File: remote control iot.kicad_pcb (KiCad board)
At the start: 2 copper layers, 97 x 122.5 mm, 13 parts, among them K1 Fujitsu_FTR-LYAA005x, Q1 BC547, SW2 SW_Push, U1 Olimex_MOD-WIFI-ESP8266-DEV, U2 AMS1117-3.3

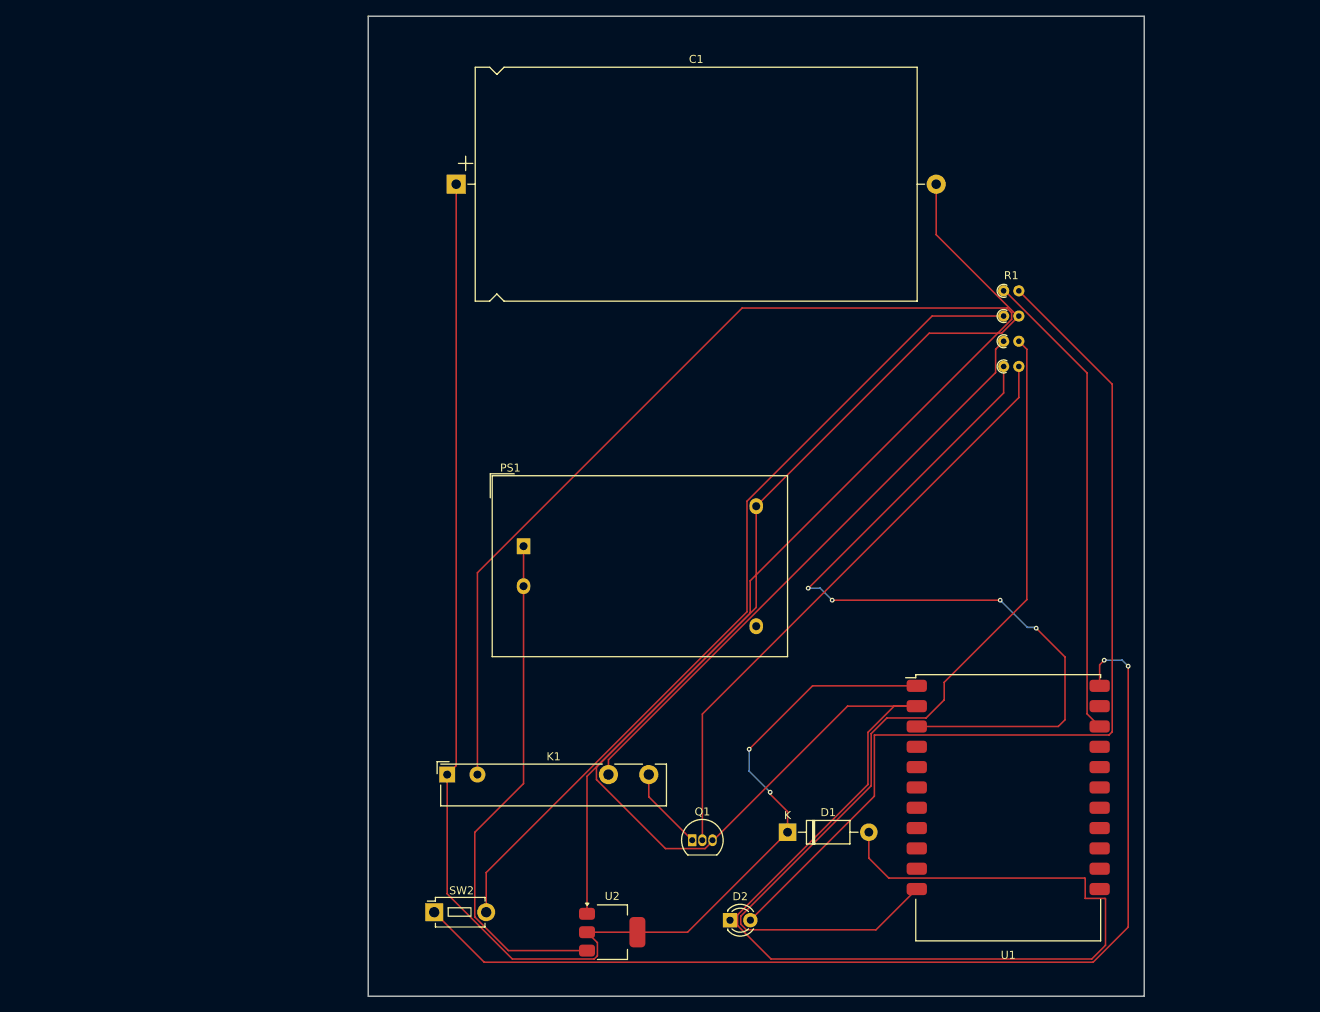
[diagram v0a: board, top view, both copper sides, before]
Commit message: Add files via upload
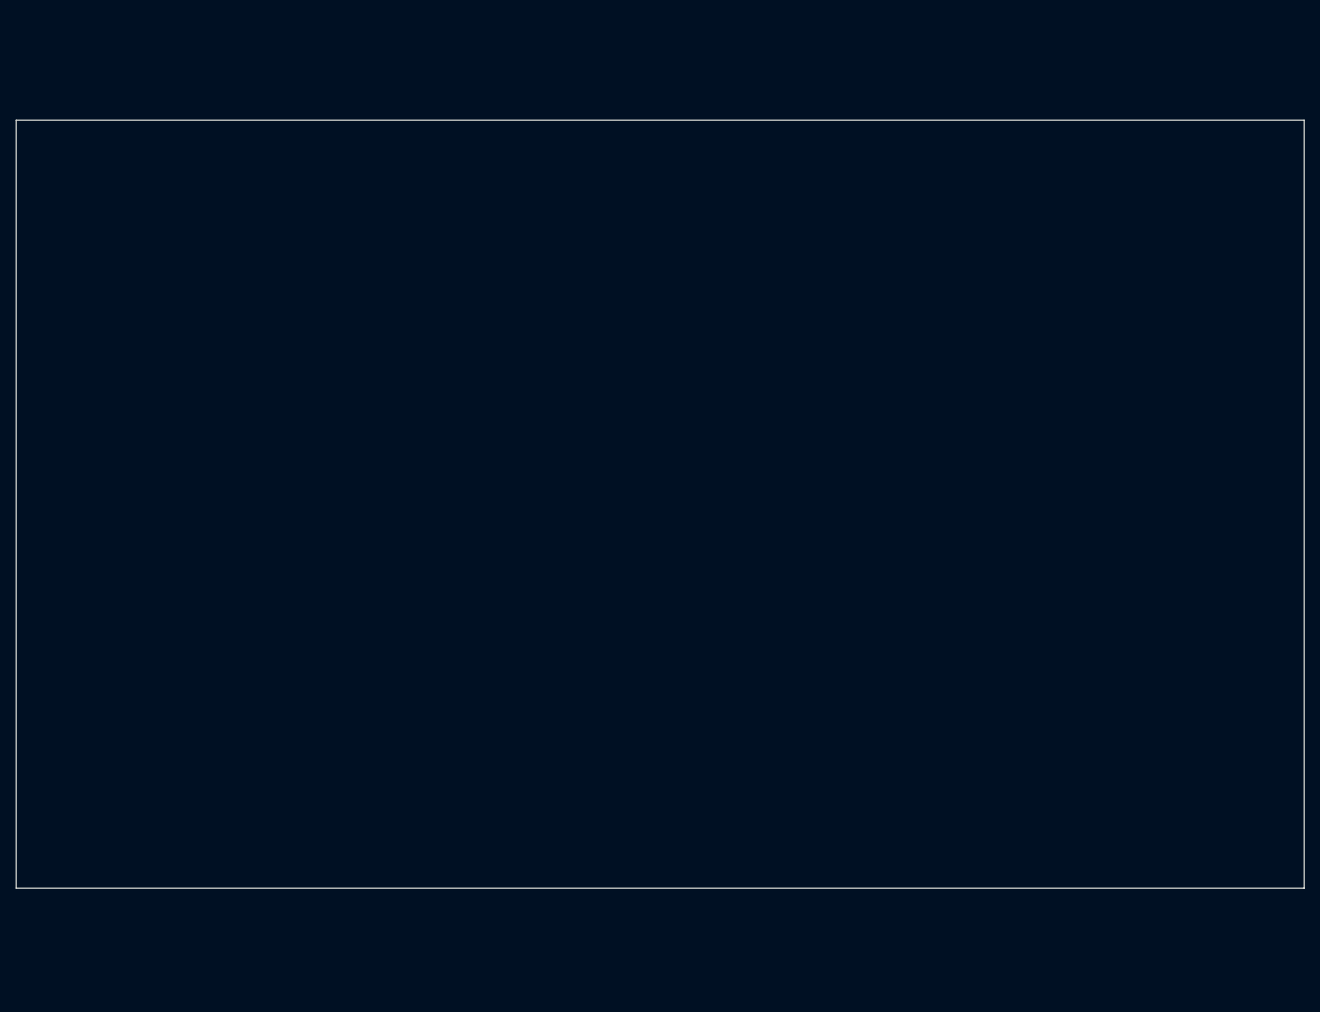
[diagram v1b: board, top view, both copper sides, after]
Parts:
- removed C1: C, Capacitor_THT:CP_Axial_L55.0mm_D29.0mm_P60.00mm_Horizontal
- removed D1: 1N4007, Diode_THT:D_DO-41_SOD81_P10.16mm_Horizontal
- removed D2: LED, LED_THT:LED_D3.0mm
- removed K1: Fujitsu_FTR-LYAA005x, Relay_THT:Relay_SPST-NO_Fujitsu_FTR-LYAA005x_FormA_Vertical
- removed PS1: HLK-PM01, Converter_ACDC:Converter_ACDC_Hi-Link_HLK-PMxx
- removed Q1: BC547, Package_TO_SOT_THT:TO-92_Inline
- removed R1, R2, R3, R4: R, Resistor_THT:R_Axial_DIN0204_L3.6mm_D1.6mm_P1.90mm_Vertical
- removed SW2: SW_Push, Button_Switch_THT:SW_PUSH_1P1T_6x3.5mm_H4.3_APEM_MJTP1243
- removed U1: Olimex_MOD-WIFI-ESP8266-DEV, Module:Olimex_MOD-WIFI-ESP8266-DEV
- removed U2: AMS1117-3.3, Package_TO_SOT_SMD:SOT-223-3_TabPin2
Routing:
- net GND: track 489.0 -> 0.00 mm
- net VCC: track 182.0 -> 0.00 mm, vias 2 -> 0
- net Net-(U1-GPIO4): track 130.4 -> 0.00 mm, vias 2 -> 0
- net Net-(D2-A): track 119.4 -> 0.00 mm
- net Net-(U1-GPIO5): track 115.4 -> 0.00 mm
- net Net-(R2-Pad1): track 106.5 -> 0.00 mm
- net Net-(U1-GPIO1): track 100.2 -> 0.00 mm, vias 4 -> 0
- net Net-(Q1-B): track 75.6 -> 0.00 mm
- net Net-(K1-Pad13): track 74.6 -> 0.00 mm
- net AC: track 64.6 -> 0.00 mm
- net Net-(U1-GPIO-2): track 59.5 -> 0.00 mm
- net Net-(Q1-C): track 10.5 -> 0.00 mm
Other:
- board size 97 x 122.5 mm -> 161 x 96 mm
